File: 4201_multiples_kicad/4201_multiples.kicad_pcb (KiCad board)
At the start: 2 copper layers, 60 x 110 mm, 73 parts, among them J1 AudioJack2, J10 Conn_01x04_Female, J11 Conn_01x05_Female, J12 Conn_01x04_Female, J13 Conn_01x04_Female, J14 Conn_01x05_Male, J15 Conn_01x04_Male, J16 Conn_01x05_Male, J17 Conn_01x04_Male, J18 Conn_01x04_Male, J19 Conn_02x05_Odd_Even, J2 AudioJack2, J3 AudioJack2, J4 AudioJack2, J5 AudioJack2, J6 AudioJack2, J7 AudioJack2, J8 AudioJack2, J9 Conn_01x05_Female, U1 TL074, U2 TL074

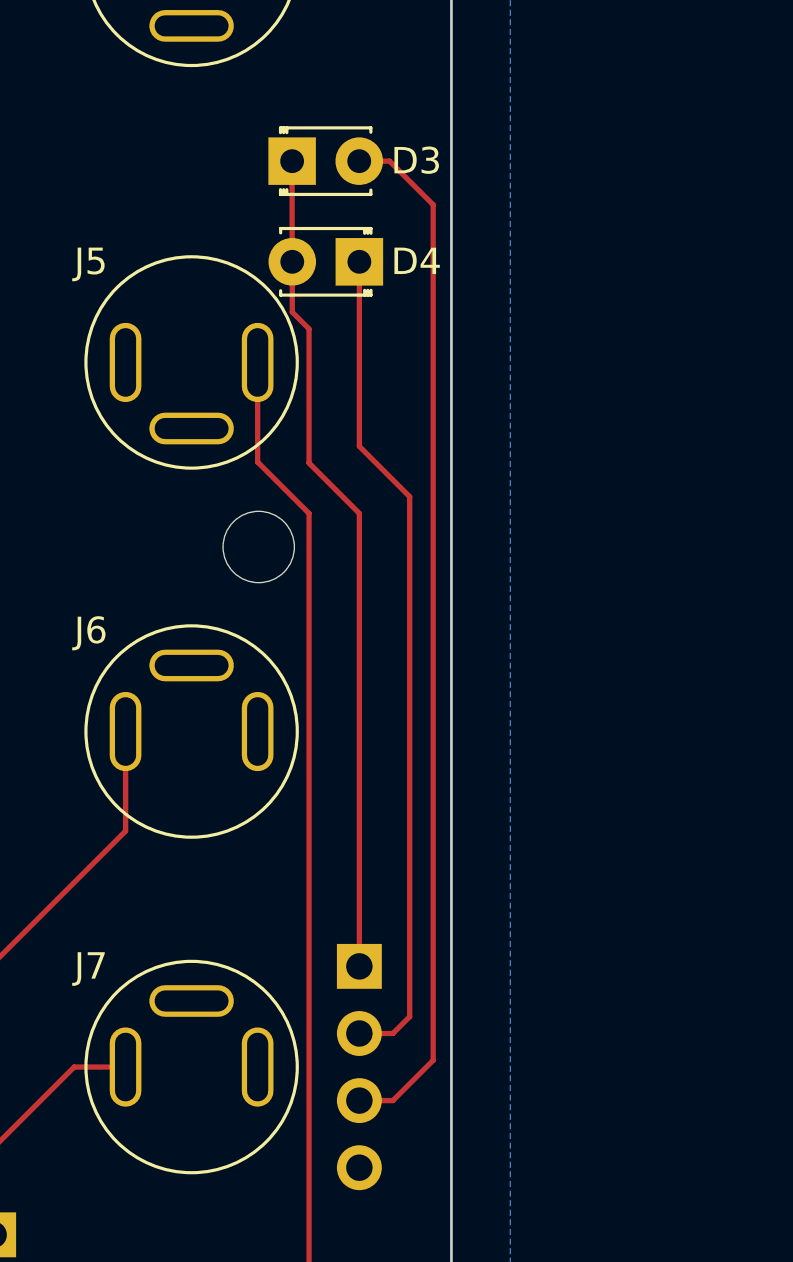
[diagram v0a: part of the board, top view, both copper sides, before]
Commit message: Small touches
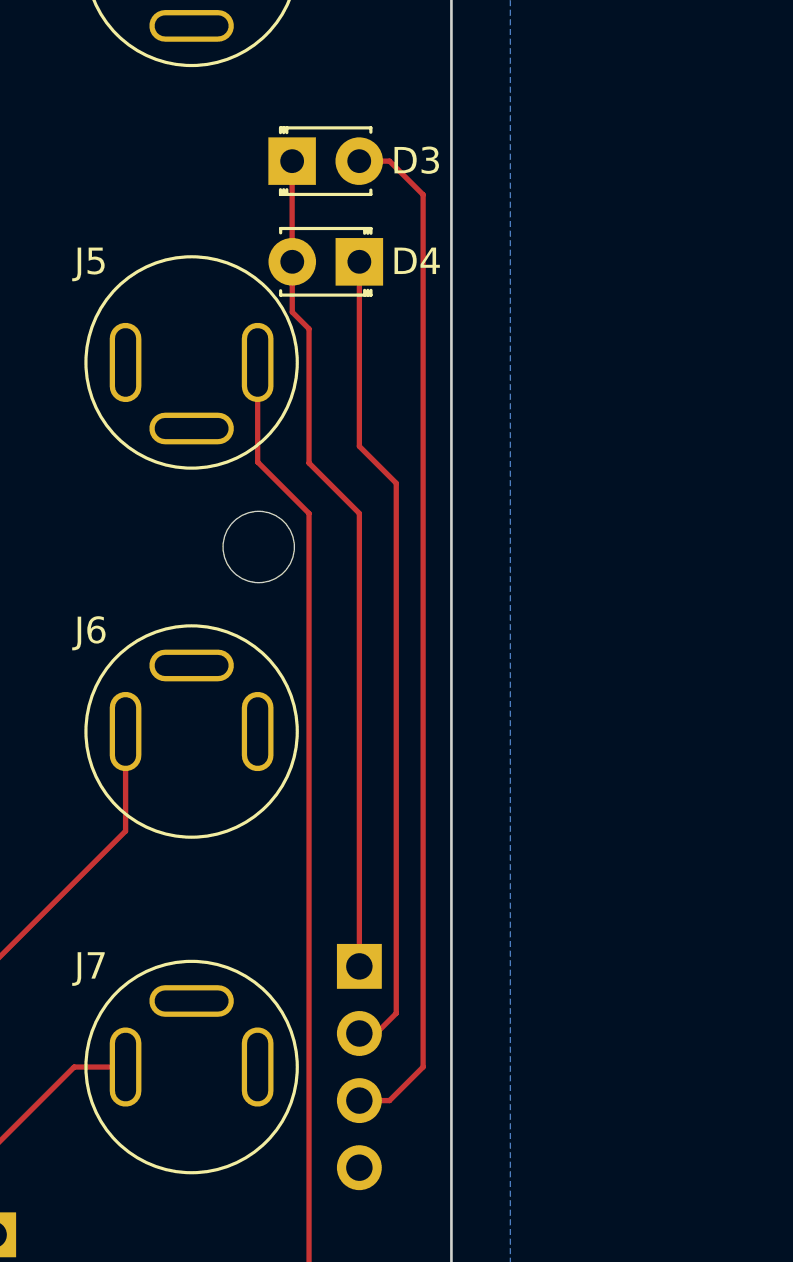
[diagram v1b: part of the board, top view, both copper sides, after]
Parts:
- D13, D14: value 1N5817 -> Schottky
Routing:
- net /interface/LED_2N_K: track 31.5 -> 30.7 mm
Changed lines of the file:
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@@
       (effects (font (size 1 1) (thickness 0.15)) (justify mirror))
     )
-    (fp_text value "1N5817" (at 0 -1.82) (layer "B.Fab") hide
+    (fp_text value "Schottky" (at 0 -1.82) (layer "B.Fab") hide
       (effects (font (size 1 1) (thickness 0.15)) (justify mirror))
     )
@@
       (effects (font (size 1 1) (thickness 0.15)) (justify mirror))
     )
-    (fp_text value "1N5817" (at 0 -1.82) (layer "B.Fab") hide
+    (fp_text value "Schottky" (at 0 -1.82) (layer "B.Fab") hide
       (effects (font (size 1 1) (thickness 0.15)) (justify mirror))
     )
@@
   (segment (start 95.885 67.31) (end 95.885 60.325) (width 0.2) (layer "F.Cu") (net 5))
   (segment (start 97.16 59.05) (end 97.16 55.88) (width 0.2) (layer "F.Cu") (net 5))
-  (segment (start 99.949 140.716) (end 99.949 108.331) (width 0.2) (layer "F.Cu") (net 6))
-  (segment (start 98.425 142.24) (end 99.949 140.716) (width 0.2) (layer "F.Cu") (net 6))
+  (segment (start 98.298 142.24) (end 99.568 140.97) (width 0.2) (layer "F.Cu") (net 6))
+  (segment (start 99.568 107.95) (end 98.298 106.68) (width 0.2) (layer "F.Cu") (net 6))
+  (segment (start 99.568 140.97) (end 99.568 107.95) (width 0.2) (layer "F.Cu") (net 6))
   (segment (start 98.298 106.68) (end 97.15 106.68) (width 0.2) (layer "F.Cu") (net 6))
-  (segment (start 97.155 142.24) (end 98.425 142.24) (width 0.2) (layer "F.Cu") (net 6))
-  (segment (start 99.949 108.331) (end 98.298 106.68) (width 0.2) (layer "F.Cu") (net 6))
-  (segment (start 97.155 139.7) (end 98.425 139.7) (width 0.2) (layer "F.Cu") (net 7))
-  (segment (start 99.06 119.38) (end 97.155 117.475) (width 0.2) (layer "F.Cu") (net 7))
-  (segment (start 98.425 139.7) (end 99.06 139.065) (width 0.2) (layer "F.Cu") (net 7))
-  (segment (start 99.06 139.065) (end 99.06 119.38) (width 0.2) (layer "F.Cu") (net 7))
+  (segment (start 97.155 142.24) (end 98.298 142.24) (width 0.2) (layer "F.Cu") (net 6))
+  (segment (start 98.552 118.872) (end 97.155 117.475) (width 0.2) (layer "F.Cu") (net 7))
+  (segment (start 98.552 138.938) (end 98.552 118.872) (width 0.2) (layer "F.Cu") (net 7))
   (segment (start 97.155 117.475) (end 97.155 110.49) (width 0.2) (layer "F.Cu") (net 7))
+  (segment (start 97.79 139.7) (end 98.552 138.938) (width 0.2) (layer "F.Cu") (net 7))
+  (segment (start 97.155 139.7) (end 97.79 139.7) (width 0.2) (layer "F.Cu") (net 7))
   (segment (start 133.8215 63.246) (end 134.874 63.246) (width 0.2) (layer "B.Cu") (net 8))
   (segment (start 135.636 64.008) (end 135.636 65.786) (width 0.2) (layer "B.Cu") (net 8))
